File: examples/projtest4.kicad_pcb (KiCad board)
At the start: 2 copper layers, 10 x 13 mm, 2 parts

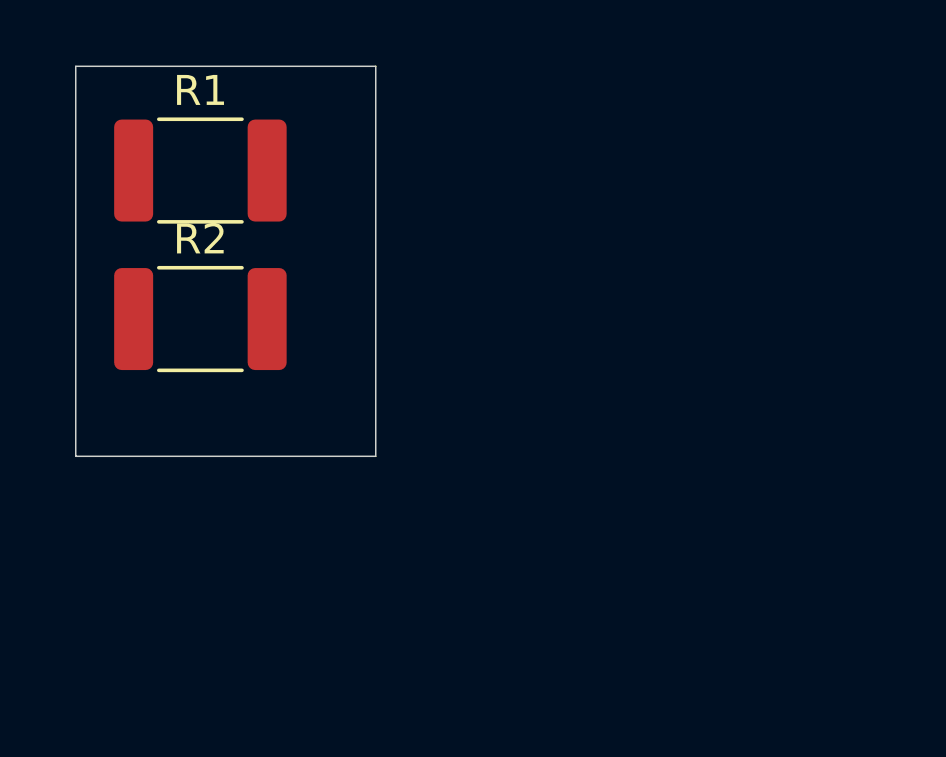
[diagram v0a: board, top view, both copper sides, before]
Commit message: First commit
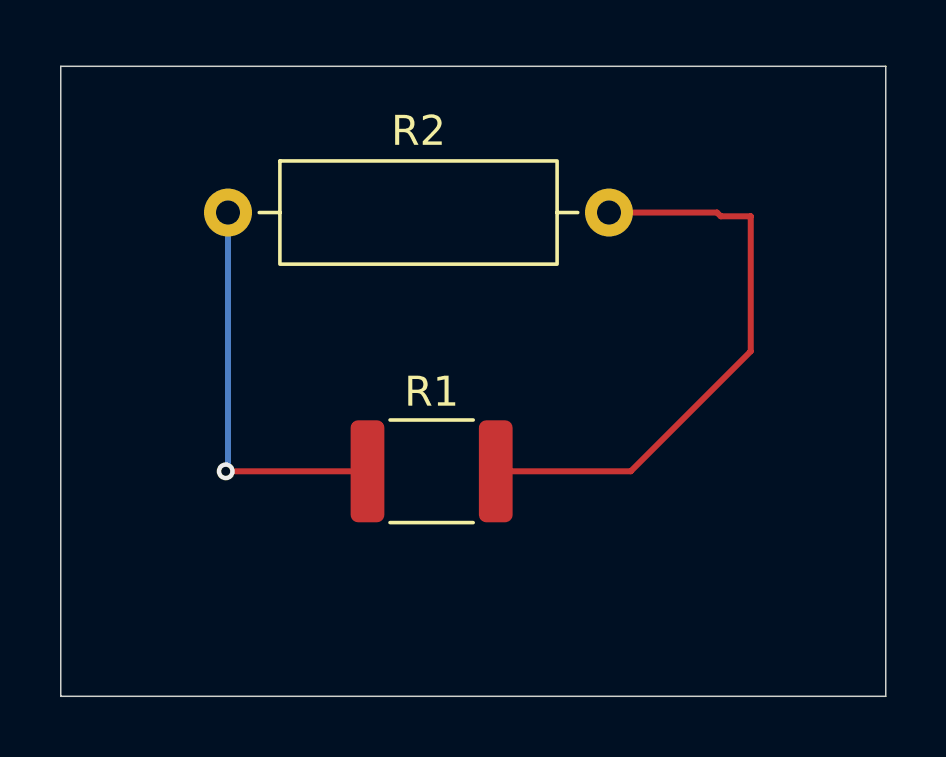
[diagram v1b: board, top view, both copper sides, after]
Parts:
- R1: footprint Resistor_SMD:R_1812_4532Metric_Pad1.30x3.40mm_HandSolder -> Resistor_SMD:R_1812_4532Metric
- R2: footprint Resistor_SMD:R_1812_4532Metric_Pad1.30x3.40mm_HandSolder -> Resistor_THT:R_Axial_DIN0309_L9.0mm_D3.2mm_P12.70mm_Horizontal
- moved R1 12.6 mm to (24.9, 26.0)
- moved R2 3.67 mm to (18.1, 17.4)
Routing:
- net Net-(R1-Pad2): track 0.00 -> 19.4 mm
- net Net-(R1-Pad1): track 0.00 -> 13.4 mm, vias 0 -> 1
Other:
- board size 10 x 13 mm -> 27.5 x 21 mm
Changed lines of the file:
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@@
 		)
 	)
-	(footprint "Resistor_SMD:R_1812_4532Metric_Pad1.30x3.40mm_HandSolder"
-		(layer "F.Cu")
-		(at 17.155 20.925)
-		(descr "Resistor SMD 1812 (4532 Metric), square (rectangular) end terminal, IPC-7351 nominal with elongated pad for handsoldering. (Body size source: https://www.nikhef.nl/pub/departments/mt/projects/detectorR_D/dtddice/ERJ2G.pdf)")
-		(tags "resistor handsolder")
-		(property "Reference" "R2"
+	(footprint "Resistor_SMD:R_1812_4532Metric"
+		(layer "F.Cu")
+		(at 24.8625 26)
+		(descr "Resistor SMD 1812 (4532 Metric), square (rectangular) end terminal, IPC-7351 nominal, (Body size source: https://www.nikhef.nl/pub/departments/mt/projects/detectorR_D/dtddice/ERJ2G.pdf)")
+		(tags "resistor")
+		(property "Reference" "R1"
 			(at 0 -2.65 0)
 			(layer "F.SilkS")
@@
 		(property ki_fp_filters "R_*")
 		(sheetname "/")
-		(sheetfile "projtest2.kicad_sch")
+		(sheetfile "projtest4.kicad_sch")
 		(units
 			(unit
@@
 		)
 		(fp_rect
-			(start -3.13 -1.95)
-			(end 3.13 1.95)
+			(start -2.95 -1.95)
+			(end 2.95 1.95)
 			(stroke
 				(width 0.05)
@@
 		)
 		(pad "1" smd roundrect
-			(at -2.225 0)
-			(size 1.3 3.4)
+			(at -2.1375 0)
+			(size 1.125 3.4)
 			(layers "F.Cu" "F.Mask" "F.Paste")
-			(roundrect_rratio 0.192308)
+			(roundrect_rratio 0.222222)
 			(net "Net-(R1-Pad1)")
 			(pintype "passive")
 		)
 		(pad "2" smd roundrect
-			(at 2.225 0)
-			(size 1.3 3.4)
+			(at 2.1375 0)
+			(size 1.125 3.4)
 			(layers "F.Cu" "F.Mask" "F.Paste")
-			(roundrect_rratio 0.192308)
+			(roundrect_rratio 0.222222)
 			(net "Net-(R1-Pad2)")
 			(pintype "passive")
@@
 		)
 	)
-	(footprint "Resistor_SMD:R_1812_4532Metric_Pad1.30x3.40mm_HandSolder"
-		(layer "F.Cu")
-		(at 17.155 15.975)
-		(descr "Resistor SMD 1812 (4532 Metric), square (rectangular) end terminal, IPC-7351 nominal with elongated pad for handsoldering. (Body size source: https://www.nikhef.nl/pub/departments/mt/projects/detectorR_D/dtddice/ERJ2G.pdf)")
-		(tags "resistor handsolder")
-		(property "Reference" "R1"
-			(at 0 -2.65 0)
+	(footprint "Resistor_THT:R_Axial_DIN0309_L9.0mm_D3.2mm_P12.70mm_Horizontal"
+		(layer "F.Cu")
+		(at 18.075 17.375)
+		(descr "Resistor, Axial_DIN0309 series, Axial, Horizontal, pin pitch=12.7mm, 0.5W = 1/2W, length*diameter=9*3.2mm^2, http://cdn-reichelt.de/documents/datenblatt/B400/1_4W%23YAG.pdf")
+		(tags "Resistor Axial_DIN0309 series Axial Horizontal pin pitch 12.7mm 0.5W = 1/2W length 9mm diameter 3.2mm")
+		(property "Reference" "R2"
+			(at 6.35 -2.72 0)
 			(layer "F.SilkS")
 			(effects
@@
 		)
 		(property "Value" "R"
-			(at 0 2.65 0)
+			(at 11.2375 6.495 0)
 			(layer "F.Fab")
 			(effects
@@
 			)
 		)
-		(property "KiLib_Generator" "SMD_2terminal_chip_molded"
+		(property "KiLib_Generator" "resistor/THT"
 			(at 0 0 0)
 			(layer "F.SilkS")
@@
 		(property ki_fp_filters "R_*")
 		(sheetname "/")
-		(sheetfile "projtest2.kicad_sch")
+		(sheetfile "projtest4.kicad_sch")
 		(units
 			(unit
@@
 			)
 		)
-		(attr smd)
+		(attr through_hole)
 		(duplicate_pad_numbers_are_jumpers no)
 		(fp_line
-			(start -1.386252 -1.71)
-			(end 1.386252 -1.71)
+			(start 1.04 0)
+			(end 1.73 0)
 			(stroke
 				(width 0.12)
@@
 		)
 		(fp_line
-			(start -1.386252 1.71)
-			(end 1.386252 1.71)
+			(start 11.66 0)
+			(end 10.97 0)
 			(stroke
 				(width 0.12)
@@
 		)
 		(fp_rect
-			(start -3.13 -1.95)
-			(end 3.13 1.95)
+			(start 1.73 -1.72)
+			(end 10.97 1.72)
+			(stroke
+				(width 0.12)
+				(type solid)
+			)
+			(fill no)
+			(layer "F.SilkS")
+		)
+		(fp_rect
+			(start -1.05 -1.85)
+			(end 13.75 1.85)
 			(stroke
 				(width 0.05)
@@
 			(layer "F.CrtYd")
 		)
+		(fp_line
+			(start 0 0)
+			(end 1.85 0)
+			(stroke
+				(width 0.1)
+				(type solid)
+			)
+			(layer "F.Fab")
+		)
+		(fp_line
+			(start 12.7 0)
+			(end 10.85 0)
+			(stroke
+				(width 0.1)
+				(type solid)
+			)
+			(layer "F.Fab")
+		)
 		(fp_rect
-			(start -2.25 -1.6)
-			(end 2.25 1.6)
+			(start 1.85 -1.6)
+			(end 10.85 1.6)
 			(stroke
 				(width 0.1)
@@
 		)
 		(fp_text user "${REFERENCE}"
-			(at 0 0 0)
-			(layer "F.Fab")
-			(effects
-				(font
-					(size 1 1)
-					(thickness 0.15)
-				)
-			)
-		)
-		(pad "1" smd roundrect
-			(at -2.225 0)
-			(size 1.3 3.4)
-			(layers "F.Cu" "F.Mask" "F.Paste")
-			(roundrect_rratio 0.192308)
+			(at 6.35 0 0)
+			(layer "F.Fab")
+			(effects
+				(font
+					(size 1 1)
+					(thickness 0.15)
+				)
+			)
+		)
+		(pad "1" thru_hole circle
+			(at 0 0)
+			(size 1.6 1.6)
+			(drill 0.8)
+			(layers "*.Cu" "*.Mask")
+			(remove_unused_layers no)
 			(net "Net-(R1-Pad1)")
 			(pintype "passive")
 		)
-		(pad "2" smd roundrect
-			(at 2.225 0)
-			(size 1.3 3.4)
-			(layers "F.Cu" "F.Mask" "F.Paste")
-			(roundrect_rratio 0.192308)
+		(pad "2" thru_hole circle
+			(at 12.7 0)
+			(size 1.6 1.6)
+			(drill 0.8)
+			(layers "*.Cu" "*.Mask")
+			(remove_unused_layers no)
 			(net "Net-(R1-Pad2)")
 			(pintype "passive")
 		)
 		(embedded_fonts no)
-		(model "${KICAD10_3DMODEL_DIR}/Resistor_SMD.3dshapes/R_1812_4532Metric.step"
+		(model "${KICAD10_3DMODEL_DIR}/Resistor_THT.3dshapes/R_Axial_DIN0309_L9.0mm_D3.2mm_P12.70mm_Horizontal.step"
 			(offset
 				(xyz 0 0 0)
@@
 	)
 	(gr_rect
-		(start 13 12.5)
-		(end 23 25.5)
+		(start 12.5 12.5)
+		(end 40 33.5)
 		(stroke
 			(width 0.05)
@@
 		(layer "Edge.Cuts")
 	)
+	(segment
+		(start 22.725 26)
+		(end 18 26)
+		(width 0.2)
+		(layer "F.Cu")
+		(net "Net-(R1-Pad1)")
+	)
+	(via
+		(at 18 26)
+		(size 0.6)
+		(drill 0.3)
+		(layers "F.Cu" "B.Cu")
+		(net "Net-(R1-Pad1)")
+	)
+	(segment
+		(start 18.075 25.925)
+		(end 18.075 17.375)
+		(width 0.2)
+		(layer "B.Cu")
+		(net "Net-(R1-Pad1)")
+	)
+	(segment
+		(start 18 26)
+		(end 18.075 25.925)
+		(width 0.2)
+		(layer "B.Cu")
+		(net "Net-(R1-Pad1)")
+	)
+	(segment
+		(start 35.5 22)
+		(end 35.5 17.5)
+		(width 0.2)
+		(layer "F.Cu")
+		(net "Net-(R1-Pad2)")
+	)
+	(segment
+		(start 31.5 26)
+		(end 35.5 22)
+		(width 0.2)
+		(layer "F.Cu")
+		(net "Net-(R1-Pad2)")
+	)
+	(segment
+		(start 35.5 17.5)
+		(end 34.5 17.5)
+		(width 0.2)
+		(layer "F.Cu")
+		(net "Net-(R1-Pad2)")
+	)
+	(segment
+		(start 34.375 17.375)
+		(end 30.775 17.375)
+		(width 0.2)
+		(layer "F.Cu")
+		(net "Net-(R1-Pad2)")
+	)
+	(segment
+		(start 34.5 17.5)
+		(end 34.375 17.375)
+		(width 0.2)
+		(layer "F.Cu")
+		(net "Net-(R1-Pad2)")
+	)
+	(segment
+		(start 27 26)
+		(end 31.5 26)
+		(width 0.2)
+		(layer "F.Cu")
+		(net "Net-(R1-Pad2)")
+	)
 	(embedded_fonts no)
